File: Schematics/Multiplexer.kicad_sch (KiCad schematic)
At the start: 101 parts, among them J10 Conn_01x02, J11 Conn_01x02, J12 Conn_01x02, J13 Conn_01x02, J14 Conn_01x02, J15 Conn_01x02, J16 Conn_01x02, J17 Conn_01x02, J5 Conn_01x02, J6 Conn_01x03, J7 Conn_01x02, J8 Conn_01x02, J9 Conn_01x02, U10 DG212C, U11 DG212C, U12 DG212C, U13 DG212C, U14 DG212C, U15 DG212C, U5 DG212C, U6 DG212C, U7 DG212C, U8 DG212C, U9 DG212C

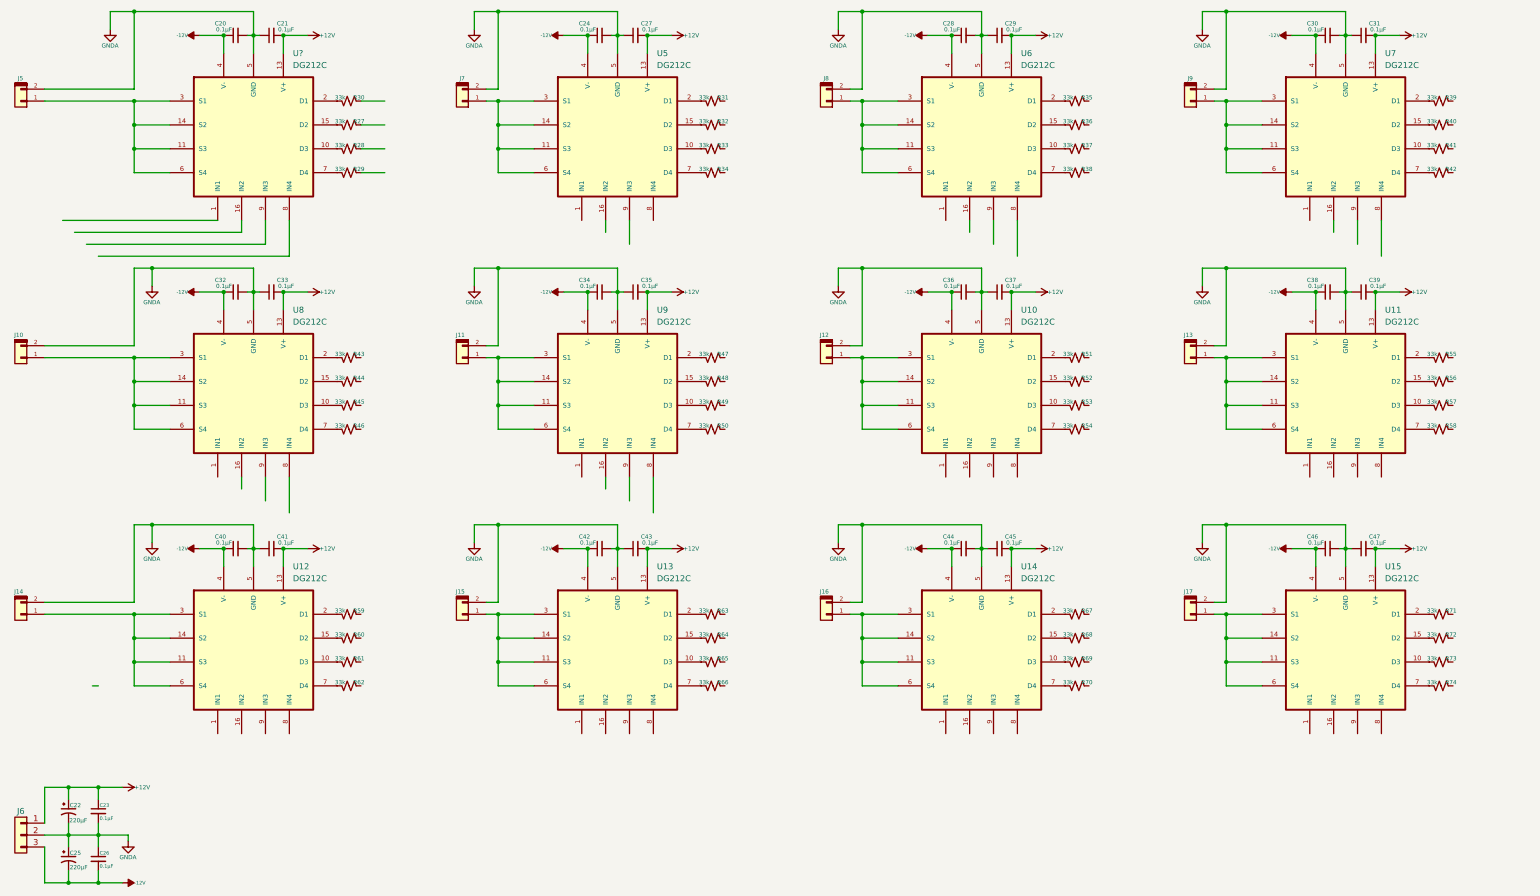
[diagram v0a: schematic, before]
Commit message: updated schematics.
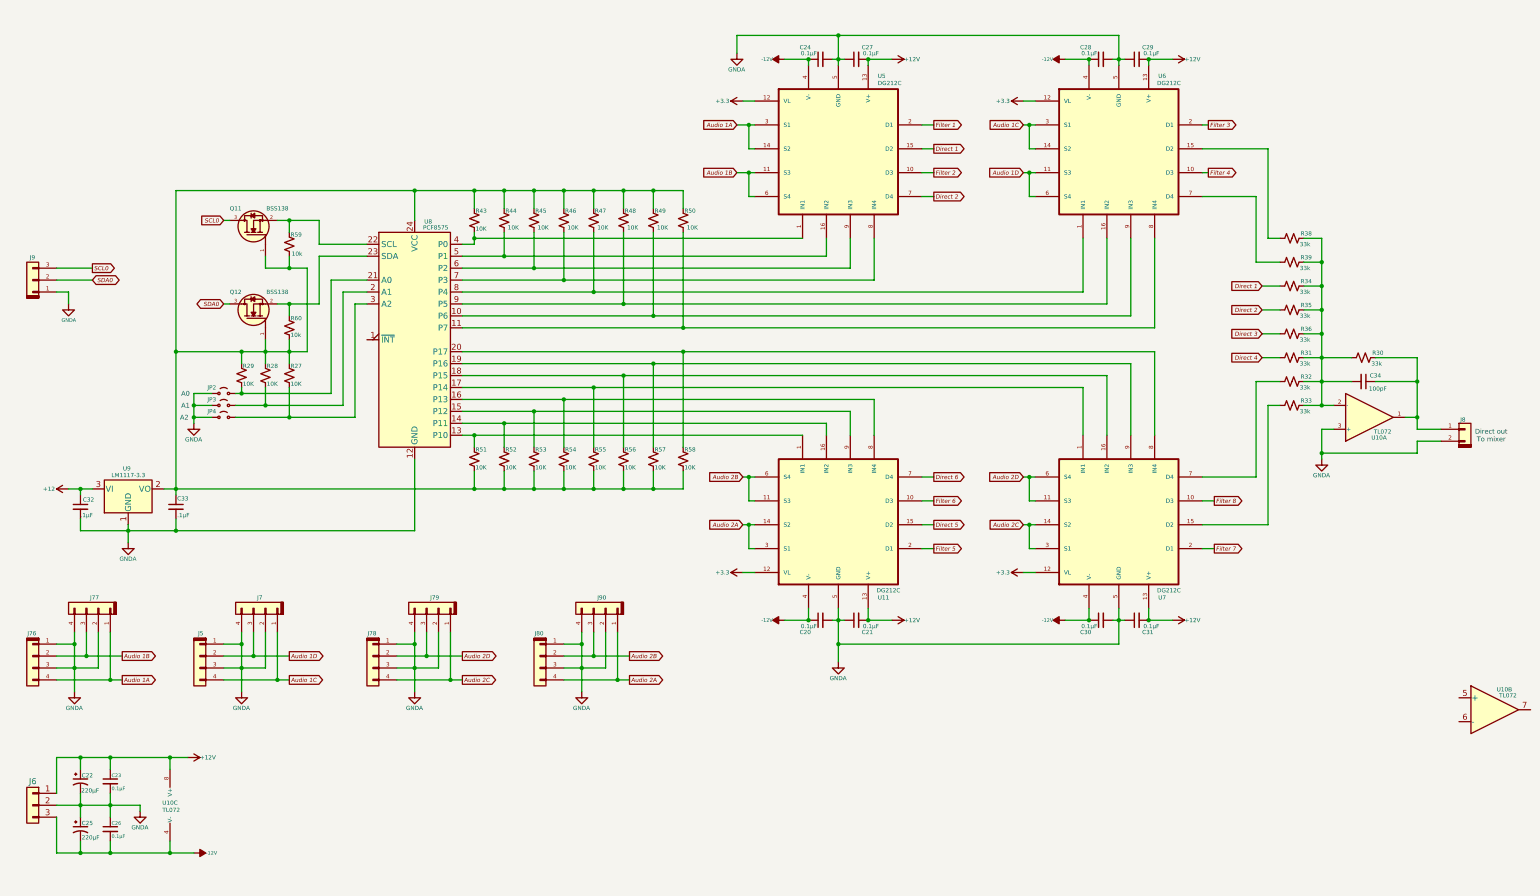
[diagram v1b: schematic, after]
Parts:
- removed C34, C35, C36, C37, C38, C39, C40, C41, C42, C43, C44, C45, C46, C47: 0.1µF, symbol Device:C_Small
- removed J10, J11, J12, J13, J14, J15, J16, J17, J5, J7, J9: Conn_01x02, symbol My Connectors:Conn_01x02
- removed R37, R40, R41, R42, R61, R62, R63, R64, R65, R66, R67, R68, R69, R70, R71, R72, R73, R74: 33k, symbol Device:R_Small_US
- removed U10, U12, U13, U14, U15, U8, U9, U?: DG212C, symbol My Chips:DG212C
- added C34: 100pF, symbol Resistors:C_Small
- added J5, J7, J76, J77, J78, J79, J80, J90: Conn_01x04, symbol My Connectors:Conn_01x04
- added J9: Conn_01x03, symbol My Connectors:Conn_01x03
- added JP2, JP3, JP4: Jumper_2_Small_Open, symbol Jumper:Jumper_2_Small_Open
- added Q11, Q12: BSS138, digikey-footprints:SOT-23-3, symbol dk_Transistors-FETs-MOSFETs-Single:BSS138
- added U10: TL072, symbol Amplifier_Operational:TL072
- added U8: PCF8575, Package_SO:SSOP-24_5.3x8.2mm_P0.65mm, symbol Interface_Expansion:PCF8575DBR
- added U9: LM1117-3.3, symbol Regulator_Linear:LM1117-3.3
- C32, C33: value 0.1µF -> .1µF
- R27, R28, R29, R43, R44, R45, R46, R47, R48, R49, R50, R51, R52, R53, R54, R55, R56, R57, R58: value 33k -> 10K
- R59, R60: value 33k -> 10k
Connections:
- net +12V: now also U10.8 (V+); no longer C33.2
- net -12V: now also U10.4 (V-); no longer C32.1
- net GNDA: now also C33.2, J5.1 (Pin_1), J5.3 (Pin_3), J7.2 (Pin_2), J7.4 (Pin_4), J76.1 (Pin_1), J76.3 (Pin_3), J77.2 (Pin_2), J77.4 (Pin_4), J78.1 (Pin_1), J78.3 (Pin_3), J79.2 (Pin_2), J79.4 (Pin_4), J80.1 (Pin_1), J80.3 (Pin_3), J9.1 (Pin_1), J90.2 (Pin_2), J90.4 (Pin_4), JP2.1 (A), JP3.1 (A), JP4.1 (A), U10.3 (+), U8.12 (GND), U9.1 (GND); no longer C33.1
- net at U7.7 (D4): now also R32.1
- net at R28.2: now also JP3.2 (B), U8.2 (A1)
- net at R27.2: now also JP4.2 (B), U8.3 (A2)
- net at R30.2: now also J8.1 (Pin_1), C34.1, U10.1
- net at R29.2: now also JP2.2 (B), U8.21 (A0)
- net at U7.15 (D2): now also R33.1
- net at R58.1: now also U7.8 (IN4), U8.20 (P17)
- net at R58.2: now also C33.1, R27.1, R28.1, R29.1, R43.1, R44.1, R45.1, R46.1, R47.1, R48.1, R49.1, R50.1, R51.2, R52.2, R53.2, R54.2, R55.2, R56.2, R57.2, R59.2, R60.2, Q11.1, Q12.1, U8.24 (VCC), U9.2 (VO); no longer U11.7 (D4)
- net at R51.1: now also U11.1 (IN1), U8.13 (P10)
- net at R49.2: now also U6.9 (IN3), U8.10 (P6)
- net at R56.1: now also U7.16 (IN2), U8.18 (P15)
- net Direct 5: now reaches U11.15 (D2)
- net Direct 5: no longer R56.2
- net at R46.2: now also U5.8 (IN4), U8.7 (P3)
- net at R53.1: now also U11.9 (IN3), U8.15 (P12)
- net Direct 2: now reaches R35.1
- net Direct 2: now also U5.7 (D4)
- net at R35.2: now also R30.1, R31.2, R32.2, R33.2, R34.2, R36.2, R38.2, R39.2, C34.2, U10.2 (-); no longer U6.2 (D1)
- net at R60.1: now also Q12.2, U8.23 (SDA)
- net at R43.2: now also U5.1 (IN1), U8.4 (P0)
- net Direct 1: now reaches R34.1
- net Direct 1: now also U5.15 (D2)
- net Audio 1A: now reaches U5.14 (S2), U5.3 (S1)
- net Audio 1A: now also J76.4 (Pin_4), J77.1 (Pin_1); no longer U5.11 (S3), U5.6 (S4)
- net Direct 3: now reaches R36.1
- net at U6.15 (D2): now also R38.1; no longer R36.2
- net at R52.1: now also U11.16 (IN2), U8.14 (P11)
- net at R48.2: now also U6.16 (IN2), U8.9 (P5)
- net at R47.2: now also U6.1 (IN1), U8.8 (P4)
- net at R50.2: now also U6.8 (IN4), U8.11 (P7)
- net at R45.2: now also U5.9 (IN3), U8.6 (P2)
- net at R44.2: now also U5.16 (IN2), U8.5 (P1)
- net Filter 4: now reaches U6.10 (D3)
- net Filter 2: now reaches U5.10 (D3)
- net Filter 2: no longer R33.2
- net Filter 1: now reaches U5.2 (D1)
- net Filter 1: no longer R31.2
- net Filter 8: now reaches U7.10 (D3)
- net Filter 6: now reaches U11.10 (D3)
- net Filter 6: no longer R57.2
- net Audio 2A: now reaches U11.14 (S2), U11.3 (S1)
- net Audio 2A: now also J80.4 (Pin_4), J90.1 (Pin_1); no longer U11.11 (S3), U11.6 (S4)
- net Filter 5: now reaches U11.2 (D1)
- net Filter 5: no longer R55.2
- net at U11.8 (IN4): now also R54.1, U8.16 (P13)
- net at R39.1: now also U6.7 (D4)
- net Filter 7: now reaches U7.2 (D1)
- net Filter 7: no longer R39.2
- net at R57.1: now also U7.9 (IN3), U8.19 (P16)
- net Direct 4: now reaches R31.1
- net at R55.1: now also U7.1 (IN1), U8.17 (P14)
- net at R59.1: now also Q11.2, U8.22 (SCL)
- net Audio 2C: now reaches U7.14 (S2), U7.3 (S1)
- net Audio 2C: now also J78.4 (Pin_4), J79.1 (Pin_1); no longer U7.11 (S3), U7.6 (S4)
- new net +12: C32.1, U9.3 (VI)
- new net +3.3: U11.12 (VL), U5.12 (VL), U6.12 (VL), U7.12 (VL)
- new net Audio 1B: J76.2 (Pin_2), J77.3 (Pin_3), U5.11 (S3), U5.6 (S4)
- new net Audio 1C: J5.4 (Pin_4), J7.1 (Pin_1), U6.14 (S2), U6.3 (S1)
- new net Audio 1D: J5.2 (Pin_2), J7.3 (Pin_3), U6.11 (S3), U6.6 (S4)
- new net Audio 2B: J80.2 (Pin_2), J90.3 (Pin_3), U11.11 (S3), U11.6 (S4)
- new net Audio 2D: J78.2 (Pin_2), J79.3 (Pin_3), U7.11 (S3), U7.6 (S4)
- new net Direct 6: U11.7 (D4)
- new net Filter 3: U6.2 (D1)
- new net SCL0: J9.3 (Pin_3), Q11.3
- new net SDA0: J9.2 (Pin_2), Q12.3
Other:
- note added: "A0"
- note added: "A1"
- note added: "A2"
- note added: "Direct out To mixer"
- moved on the sheet: C20, C21, C22, C23, C24, C25, C26, C27, C28, C29, C30, C31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
